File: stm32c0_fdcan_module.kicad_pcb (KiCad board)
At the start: 2 copper layers, 28 x 26.5 mm, 32 parts, among them IC1 STM32C092GCU6, IC2 TJA1051TK_3,118, J1 12505WS-04, J2 Conn_01x10, J3 Conn_01x10, J4 12505WS-06, SW1 DSHP02TSGER, U1 XC6206P332MR, Y1 8MHz_50X32mm

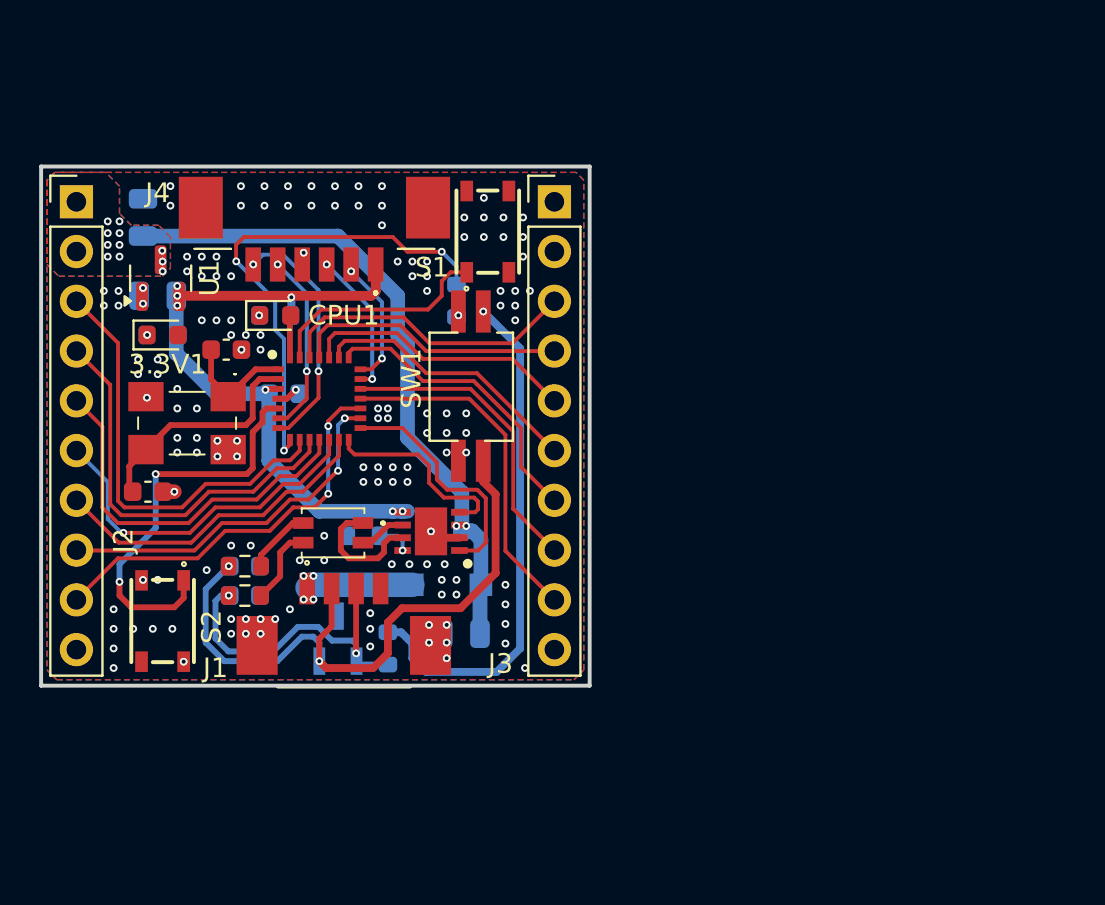
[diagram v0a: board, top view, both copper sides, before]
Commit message: 단면 배치 버전
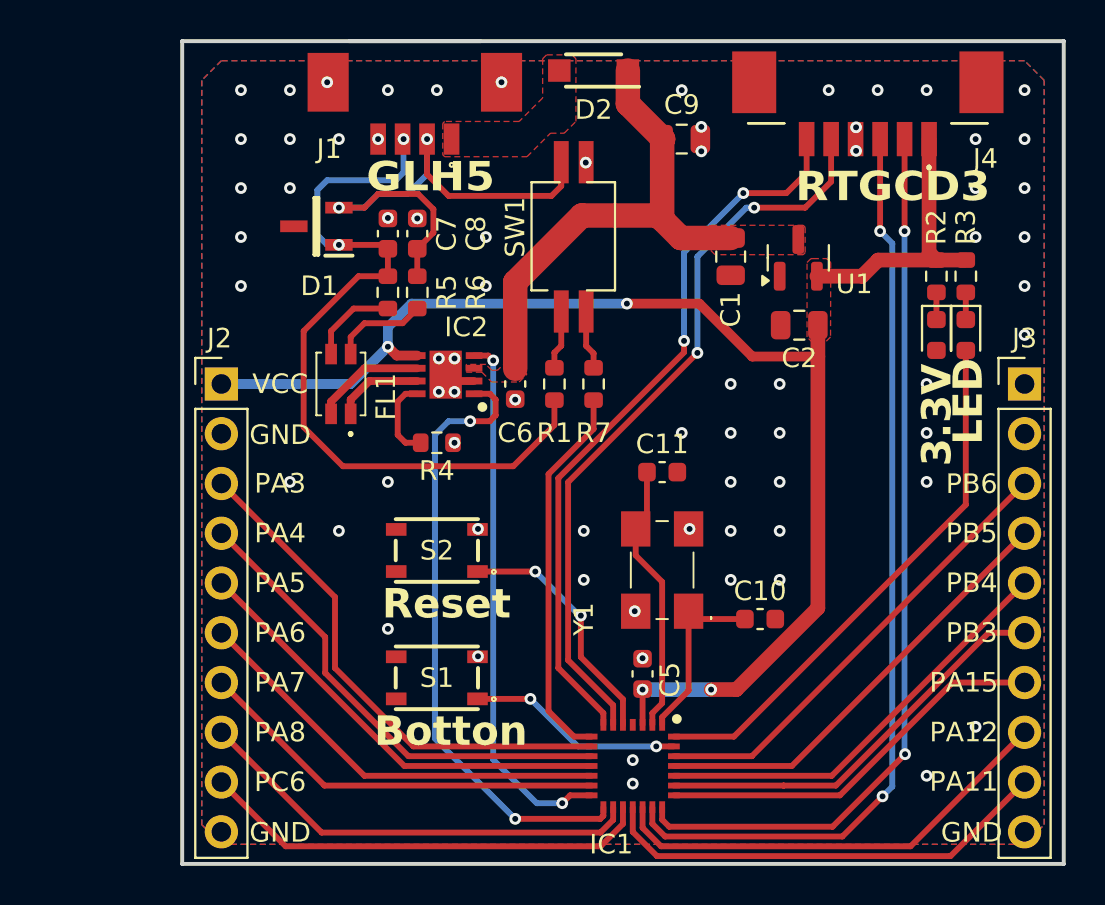
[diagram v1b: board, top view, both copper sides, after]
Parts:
- C1, C2, C5, C6, C7, C8, C9, D1, D2, R1, R2, R3, R4, R7: moved to F.Cu
- moved R2 39.6 mm to (140.5, 82.0), turned to 90 degrees
- moved 3.3V1 39.5 mm to (140.5, 85.0), turned to -90 degrees
- moved R3 35.3 mm to (142.0, 82.0), turned to 90 degrees
- moved CPU1 35.3 mm to (142.0, 85.0), turned to -90 degrees
- moved C2 32.8 mm to (133.5, 84.5)
- moved U1 32.6 mm to (133.4, 81.1)
- moved C10 30.5 mm to (131.5, 99.5)
- moved C1 30.1 mm to (130.0, 81.0), turned to -90 degrees
- moved J4 29.0 mm to (137.0, 72.1)
- moved C9 27.6 mm to (127.5, 75.0), turned to 0 degrees
- moved D2 27.3 mm to (123.0, 71.5)
- moved C11 26.3 mm to (126.5, 92.0)
- moved J3 25.7 mm to (145.0, 87.5)
- moved Y1 25.4 mm to (126.5, 97.0), turned to 90 degrees
- moved J1 24.8 mm to (113.9, 74.2), turned to 180 degrees
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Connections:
- J2 pad 1: 5V -> +3.3V
- J2 pad 2: 5V -> GND
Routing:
- net +3.3V: track 33.4 -> 76.7 mm, vias 7 -> 4
- net SWCLK: track 7.41 -> 47.7 mm
- net SWDIO: track 6.43 -> 46.1 mm
- net UART1_TX: track 9.33 -> 38.2 mm
- net LED: track 2.17 -> 27.7 mm
- net UART1_RX: track 12.5 -> 37.4 mm
- net Net-(R1-Pad1): track 26.5 -> 3.02 mm, vias 1 -> 0
- net CAN_L: track 16.9 -> 40.2 mm
- net FDCAN_TX: track 12.2 -> 31.8 mm, vias 0 -> 2
- net FDCAN_RX: track 10.1 -> 27.6 mm, vias 0 -> 2
- net PB5: track 13.9 -> 22.8 mm
- net PB6: track 15.5 -> 23.7 mm
- net PB4: track 14.0 -> 22.0 mm
- net nRST: track 20.6 -> 12.7 mm
- net PA12: track 15.6 -> 23.4 mm
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- added copper zone on F.Cu, net +3.3V
- added copper zone on F.Cu, net Net-(D2-A)
- removed copper zone on B.Cu, net 5V
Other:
- board size 28 x 26.5 mm -> 45 x 42 mm
- board text added: "3.3V"
- board text added: "Botton"
- board text added: "GLH5"
- board text added: "GND"
- board text added: "LED"
- board text added: "PA11"
- board text added: "PA12"
- board text added: "PA15"
- board text added: "PA3"
- board text added: "PA4"
- board text added: "PA5"
- board text added: "PA6"
- board text added: "PA7"
- board text added: "PA8"
- board text added: "PB3"
- board text added: "PB4"
- board text added: "PB5"
- board text added: "PB6"
- board text added: "PC6"
- board text added: "RTGCD3"
- board text added: "Reset"
- board text added: "VCC"
- board text removed: "25.04.27"
- board text removed: "STM32C0 FDCAN Board"
